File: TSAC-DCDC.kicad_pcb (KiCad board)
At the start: 2 copper layers, 30 parts, among them IC1 PS2811-1-A, Q2 IPB95R450PFD7ATMA1, U1 UCC28C44DR, U3 TL432DBZ

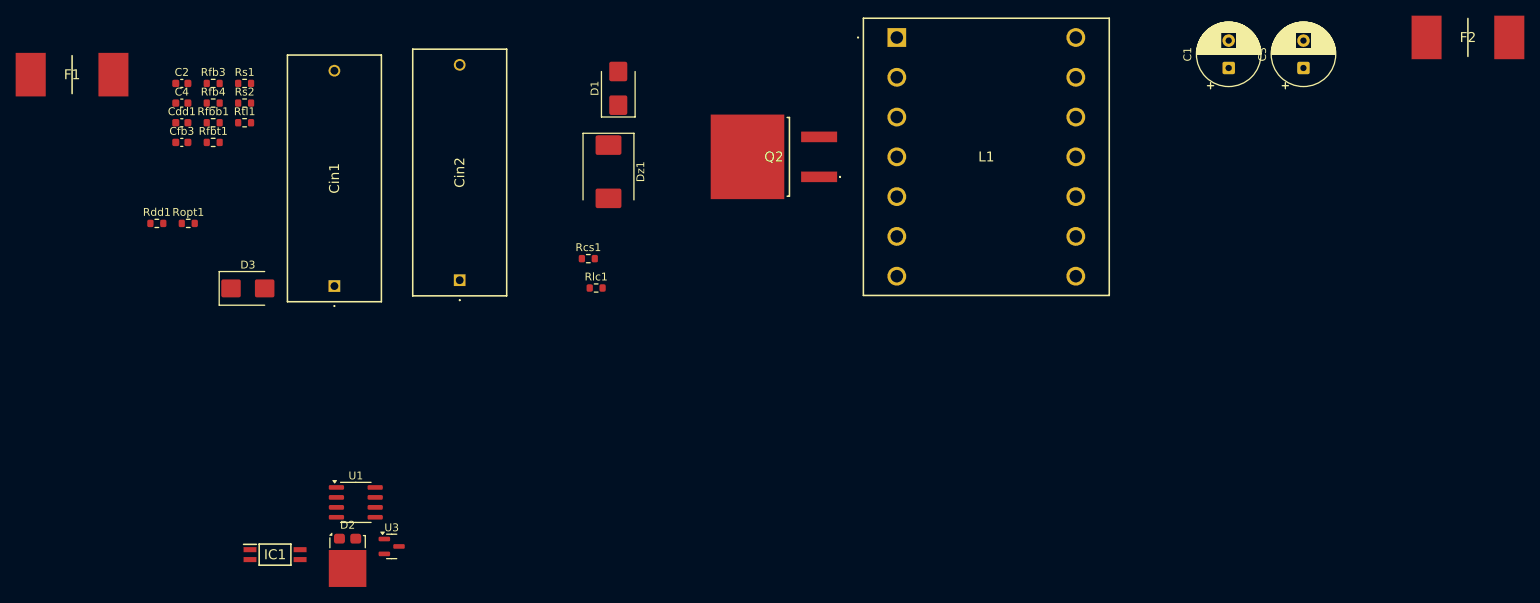
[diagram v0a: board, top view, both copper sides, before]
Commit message: Initial PCB layout
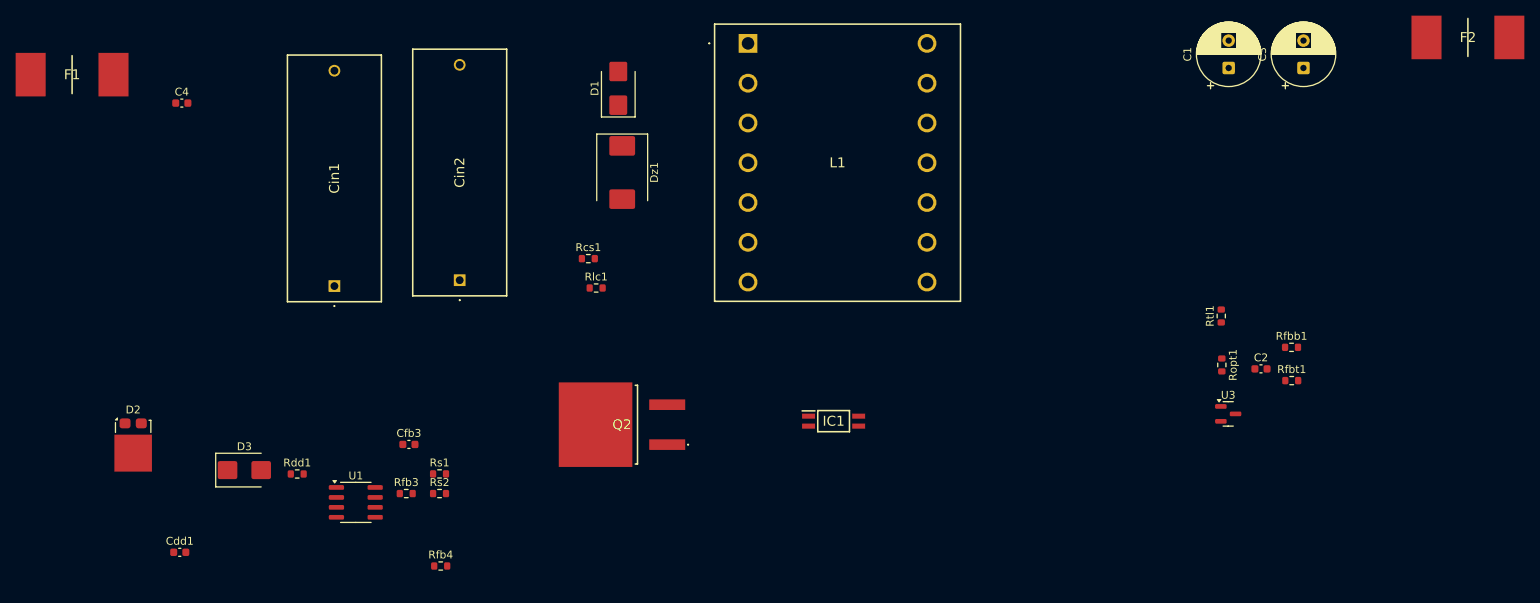
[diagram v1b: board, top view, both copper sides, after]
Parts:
- moved C2 142.6 mm to (203.1, 70.8)
- moved Rfbt1 141.0 mm to (207.0, 72.3)
- moved Rfbb1 140.7 mm to (207.0, 68.1)
- moved Ropt1 133.2 mm to (198.1, 70.3), turned to -90 degrees
- moved Rtl1 127.1 mm to (198.0, 64.1), turned to 90 degrees
- moved U3 108.2 mm to (198.9, 76.6)
- moved IC1 73.3 mm to (148.5, 77.5)
- moved Rfb4 65.9 mm to (98.3, 96.0)
- moved Rfb3 57.9 mm to (93.9, 86.8)
- moved Rs1 55.7 mm to (98.2, 84.2)
- moved Rs2 55.7 mm to (98.2, 86.8)
- moved Cdd1 54.9 mm to (65.0, 94.2)
- moved Cfb3 48.3 mm to (94.3, 80.5)
- moved Q2 39.3 mm to (119.0, 78.0)
- moved Rdd1 36.7 mm to (80.0, 84.2)
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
